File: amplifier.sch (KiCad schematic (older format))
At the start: 27 parts, among them J2 J_3.5mm_jack_SJ1-3523N, J3 J_2_screwterminal_2.54_282834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, Q1 Q_IRFZ44NPBF_N-Channel_Infine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, Q2 Q_IRFZ44NPBF_N-Channel_Infine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, U2 U_LM358AP_TI_DIP, U3 U_LM393N_NOPB, U4 U_TC4427M_Microchip

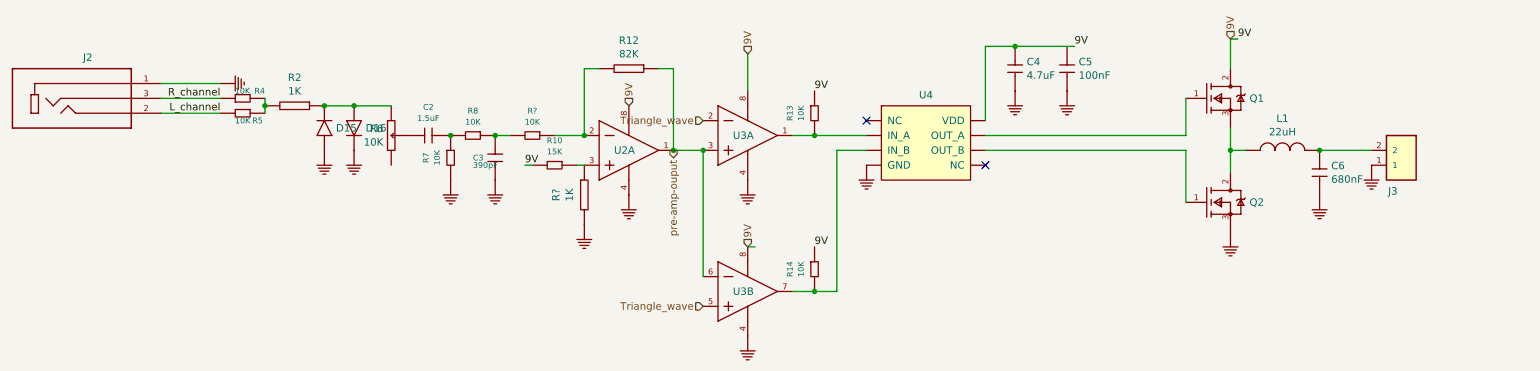
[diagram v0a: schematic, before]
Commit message: no message
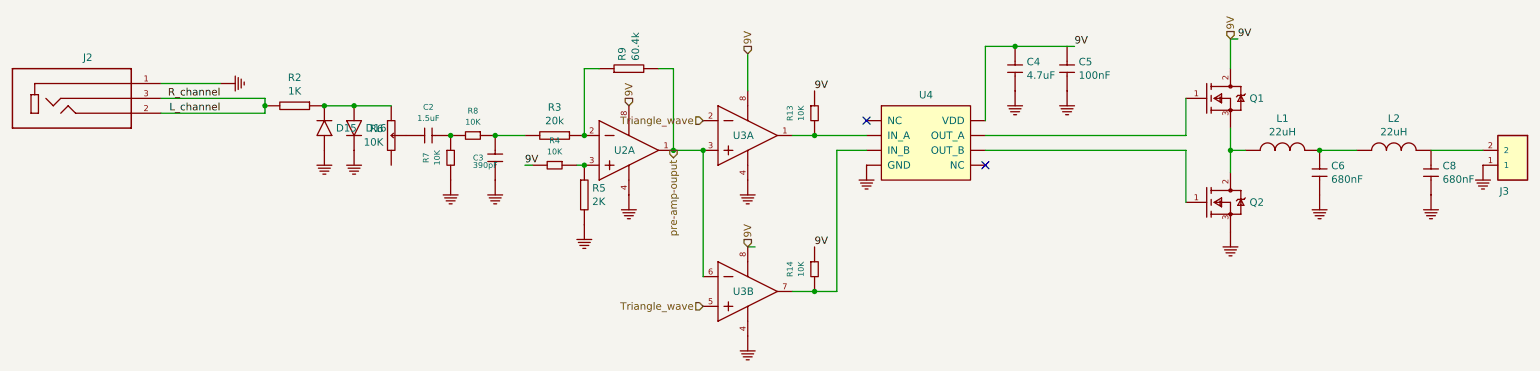
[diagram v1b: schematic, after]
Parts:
- removed R10, R5, R?: R_10K_0603, MAIN_PCB_LIB:R_0603, symbol Main_Library:R_10K_0603
- removed R12: R_60.4K_0603, MAIN_PCB_LIB:R_0603, symbol Main_Library:R_60.4K_0603
- removed R?: R_1K_0603, MAIN_PCB_LIB:R_0603, symbol Main_Library:R_1K_0603
- added C8: C_680nF_TH_450V, MAIN_PCB_LIB:C_ECWFD_Panasonic, symbol Main_Library:C_680nF_TH_450V
- added L2: L_22uH_RFS1113_coilcraft_TH, MAIN_PCB_LIB:L_RFS1113_coilcraft, symbol Main_Library:L_22uH_RFS1113_coilcraft_TH
- added R3: R_20K_0603, MAIN_PCB_LIB:R_0603, symbol Main_Library:R_20K_0603
- added R5: R_2K_0603, MAIN_PCB_LIB:R_0603, symbol Main_Library:R_2K_0603
- added R9: R_60.4K_0603, MAIN_PCB_LIB:R_0603, symbol Main_Library:R_60.4K_0603
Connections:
- net 9V: now also R4.2
- net L_channel: now also J2.3, R2.2
- net pre-amp-ouput: now also R9.2
- net at C3.1, R8.1: now also R3.2
- net at C6.1, L1.2: now also L2.1; no longer J3.2
- net at U2.2 (1IN-): now also R3.1, R9.1
- net at U2.3 (1IN+): now also R4.1, R5.1
- removed net R_channel: J2.3, R4.1
- new net: C8.1, J3.2, L2.2
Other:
- moved on the sheet: J3
